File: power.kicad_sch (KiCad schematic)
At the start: 31 parts, among them J501 694106301002, U501 LMR50410, U502 TLV1117-50, U503 TLV74133PDBVR

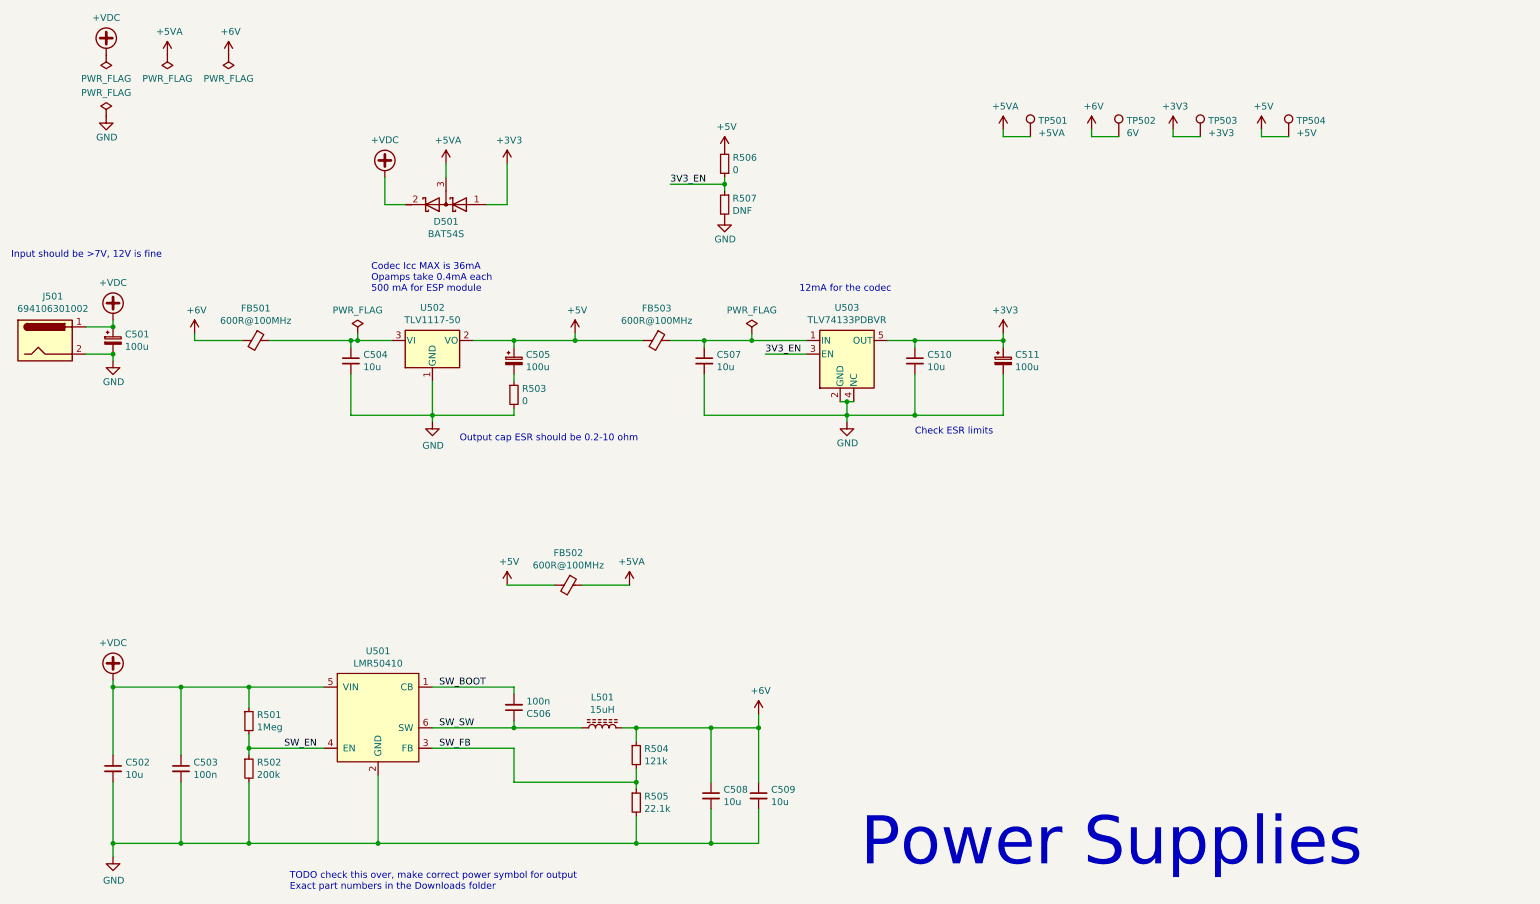
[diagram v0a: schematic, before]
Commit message: Working on schematic
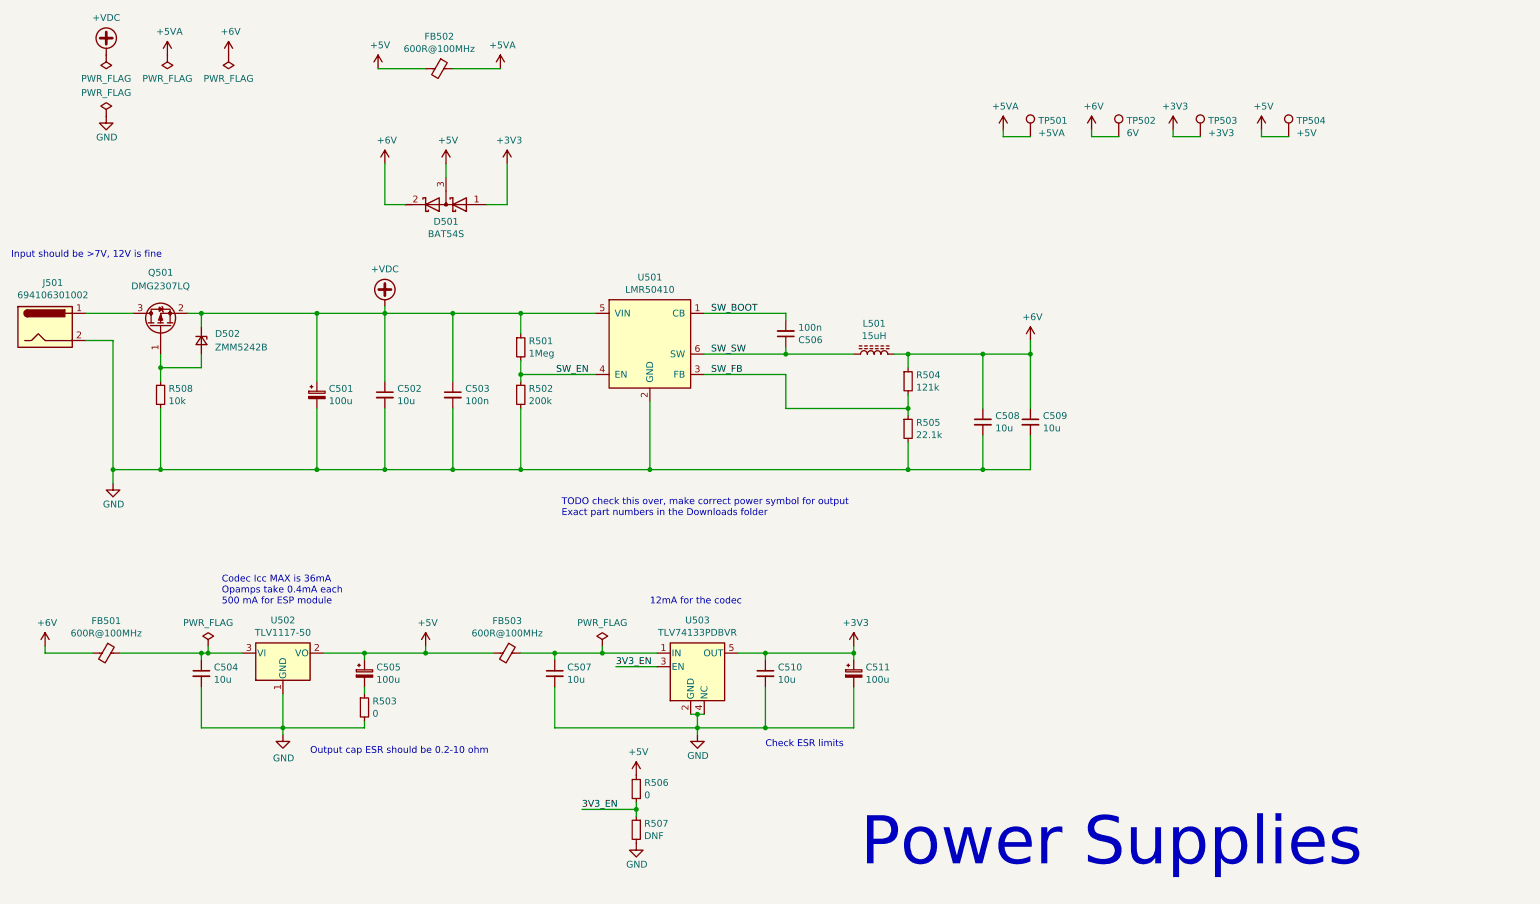
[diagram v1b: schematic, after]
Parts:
- added D502: ZMM5242B, Diode_SMD:D_MiniMELF, symbol Device:D_Zener_Small
- added Q501: DMG2307LQ, Package_TO_SOT_SMD:SOT-23, symbol Device:Q_PMOS_GSD
- added R508: 10k, Resistor_SMD:R_0805_2012Metric_Pad1.20x1.40mm_HandSolder, symbol Device:R_Small
- C503, C506: footprint (none) -> Capacitor_SMD:C_0805_2012Metric_Pad1.18x1.45mm_HandSolder
- R501, R502, R504, R505: footprint (none) -> Resistor_SMD:R_0805_2012Metric_Pad1.20x1.40mm_HandSolder
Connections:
- net +5V: now also D501.3 (common)
- net +5VA: no longer D501.3 (common)
- net +6V: now also D501.2 (K)
- net +VDC: now also D502.1 (K), Q501.2 (S); no longer D501.2 (K), J501.1
- net GND: now also R508.2
- new net: J501.1, Q501.3 (D)
- new net: D502.2 (A), Q501.1 (G), R508.1
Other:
- moved on the sheet: C501, C502, C503, C504, C505, C506, C507, C508, C509, C510, C511, FB501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
